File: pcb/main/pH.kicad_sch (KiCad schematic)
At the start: 12 parts

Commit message: fix: symbol libraries in Kicad 6.0
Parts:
- C1, C3: renamed from C?; value (none) -> 100n; footprint (none) -> Capacitor_SMD:C_0805_2012Metric_Pad1.15x1.40mm_HandSolder; symbol pHMeter-rescue:C-Device -> Device:C
- C9: renamed from C?; value (none) -> 22u; footprint (none) -> Capacitor_SMD:C_0805_2012Metric_Pad1.15x1.40mm_HandSolder; symbol pHMeter-rescue:C-Device -> Device:C
- J3: renamed from J?; symbol pHMeter-rescue:Conn_Coaxial_Power-Connector -> Connector:Conn_Coaxial_Power
- R11: renamed from R?; value (none) -> 56.2k; footprint (none) -> Resistor_SMD:R_0805_2012Metric_Pad1.15x1.40mm_HandSolder; symbol pHMeter-rescue:R-Device -> Device:R
- R13, R3, R4: renamed from R?; value (none) -> 10k; footprint (none) -> Resistor_SMD:R_0805_2012Metric_Pad1.15x1.40mm_HandSolder; symbol pHMeter-rescue:R-Device -> Device:R
- U1: renamed from U?; value (none) -> TLV6004PW; footprint (none) -> Package_SO:TSSOP-14_4.4x5mm_P0.65mm
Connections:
- net GND: now also C1.2, C3.2, C9.2, R4.2
- net Vin: now also C1.1, R3.2
- net pH+: now also C9.1, R11.1, R13.2
- net pH-: now also R13.1
- net at U1.3 (+), U1.5 (+): now also C3.1, R3.1, R4.1
- net at U1.10 (+): now also J3.1 (In)
- net at U1.8, U1.9 (-): now also R11.2
- net at U1.1, U1.2 (-): now also J3.2 (Ext)

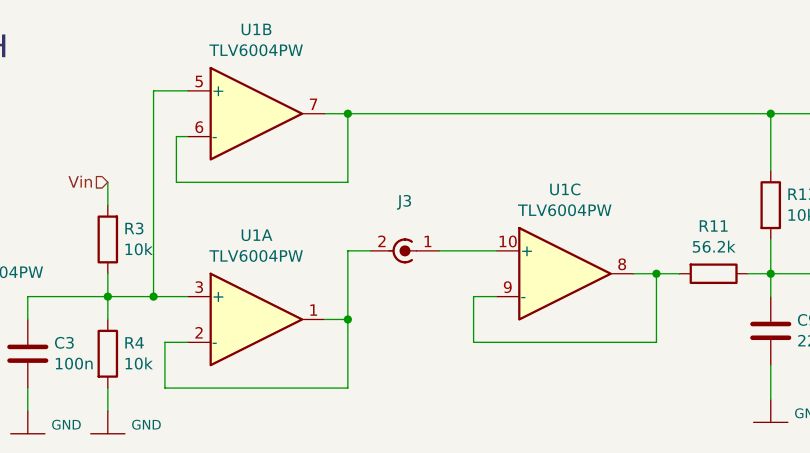
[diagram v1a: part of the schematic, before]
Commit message: fix: 3D model libraries in Kicad 6.0
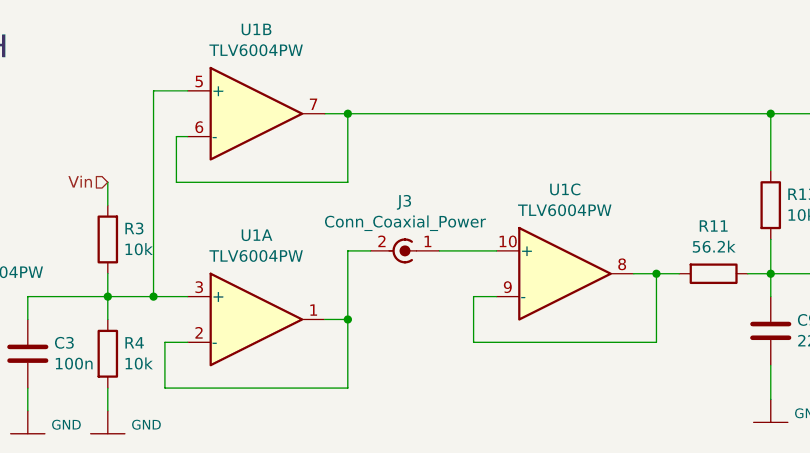
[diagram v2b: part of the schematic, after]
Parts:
- J3: value (none) -> Conn_Coaxial_Power; footprint (none) -> Connector_Coaxial:BNC_TEConnectivity_1478204_Vertical
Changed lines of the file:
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@@
     (in_bom yes) (on_board yes)
     (property "Reference" "J3" (id 0) (at 157.48 97.3582 90))
-    (property "Value" "" (id 1) (at 157.48 99.6696 90))
-    (property "Footprint" "" (id 2) (at 157.48 102.87 0)
+    (property "Value" "Conn_Coaxial_Power" (id 1) (at 157.48 99.6696 90))
+    (property "Footprint" "Connector_Coaxial:BNC_TEConnectivity_1478204_Vertical" (id 2) (at 157.48 102.87 0)
       (effects (font (size 1.27 1.27)) hide)
     )

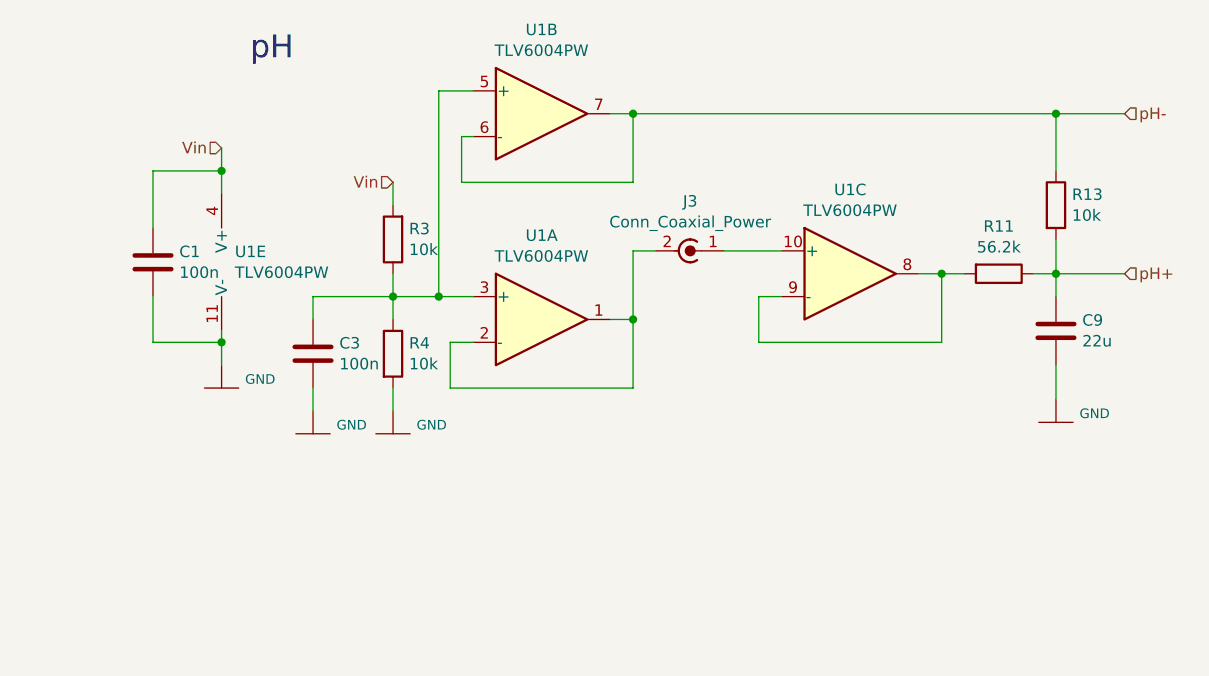
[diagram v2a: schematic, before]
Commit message: fix: standard footprint for R and C, BOM updated
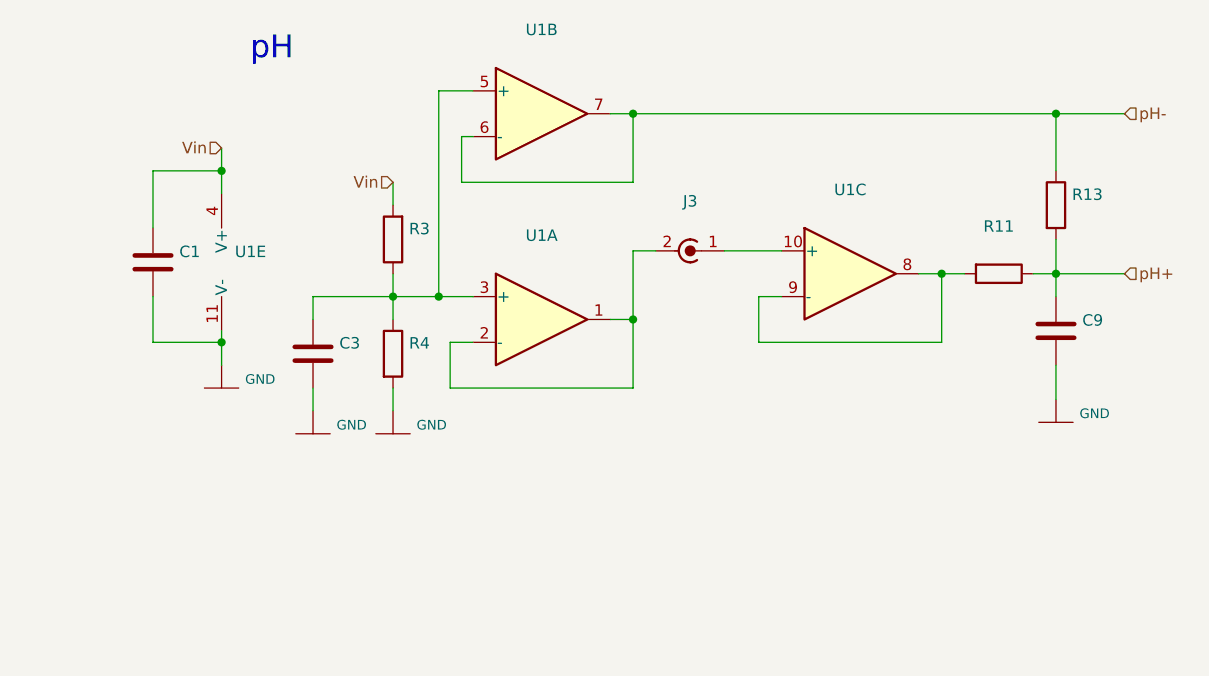
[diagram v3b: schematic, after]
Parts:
- C1, C3: value 100n -> (none); footprint Capacitor_SMD:C_0805_2012Metric_Pad1.15x1.40mm_HandSolder -> (none)
- C9: value 22u -> (none); footprint Capacitor_SMD:C_0805_2012Metric_Pad1.15x1.40mm_HandSolder -> (none)
- J3: value Conn_Coaxial_Power -> (none); footprint Connector_Coaxial:BNC_TEConnectivity_1478204_Vertical -> (none)
- R11: value 56.2k -> (none); footprint Resistor_SMD:R_0805_2012Metric_Pad1.15x1.40mm_HandSolder -> (none)
- R13, R3, R4: value 10k -> (none); footprint Resistor_SMD:R_0805_2012Metric_Pad1.15x1.40mm_HandSolder -> (none)
- U1: value TLV6004PW -> (none); footprint Package_SO:TSSOP-14_4.4x5mm_P0.65mm -> (none)
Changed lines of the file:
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@@
     (in_bom yes) (on_board yes)
     (property "Reference" "U1" (id 0) (at 140.97 78.3082 0))
-    (property "Value" "TLV6004PW" (id 1) (at 140.97 80.6196 0))
-    (property "Footprint" "Package_SO:TSSOP-14_4.4x5mm_P0.65mm" (id 2) (at 140.97 87.63 0)
+    (property "Value" "" (id 1) (at 140.97 80.6196 0))
+    (property "Footprint" "" (id 2) (at 140.97 87.63 0)
       (effects (font (size 1.27 1.27)) hide)
     )
@@
       (effects (font (size 1.27 1.27)) (justify left))
     )
-    (property "Value" "100n" (id 1) (at 118.491 115.443 0)
-      (effects (font (size 1.27 1.27)) (justify left))
-    )
-    (property "Footprint" "Capacitor_SMD:C_0805_2012Metric_Pad1.15x1.40mm_HandSolder" (id 2) (at 116.5352 118.11 0)
+    (property "Value" "" (id 1) (at 118.491 115.443 0)
+      (effects (font (size 1.27 1.27)) (justify left))
+    )
+    (property "Footprint" "" (id 2) (at 116.5352 118.11 0)
       (effects (font (size 1.27 1.27)) hide)
     )
@@
       (effects (font (size 1.27 1.27)) (justify right))
     )
-    (property "Value" "10k" (id 1) (at 126.238 102.743 0)
+    (property "Value" "" (id 1) (at 126.238 102.743 0)
       (effects (font (size 1.27 1.27)) (justify right))
     )
-    (property "Footprint" "Resistor_SMD:R_0805_2012Metric_Pad1.15x1.40mm_HandSolder" (id 2) (at 126.238 101.6 90)
+    (property "Footprint" "" (id 2) (at 126.238 101.6 90)
       (effects (font (size 1.27 1.27)) hide)
     )
@@
     (in_bom yes) (on_board yes)
     (property "Reference" "J3" (id 0) (at 157.48 97.3582 90))
-    (property "Value" "Conn_Coaxial_Power" (id 1) (at 157.48 99.6696 90))
-    (property "Footprint" "Connector_Coaxial:BNC_TEConnectivity_1478204_Vertical" (id 2) (at 157.48 102.87 0)
+    (property "Value" "" (id 1) (at 157.48 99.6696 90))
+    (property "Footprint" "" (id 2) (at 157.48 102.87 0)
       (effects (font (size 1.27 1.27)) hide)
     )
@@
     (in_bom yes) (on_board yes)
     (property "Reference" "U1" (id 0) (at 175.26 96.0882 0))
-    (property "Value" "TLV6004PW" (id 1) (at 175.26 98.3996 0))
-    (property "Footprint" "Package_SO:TSSOP-14_4.4x5mm_P0.65mm" (id 2) (at 175.26 105.41 0)
+    (property "Value" "" (id 1) (at 175.26 98.3996 0))
+    (property "Footprint" "" (id 2) (at 175.26 105.41 0)
       (effects (font (size 1.27 1.27)) hide)
     )
@@
     (in_bom yes) (on_board yes)
     (property "Reference" "R11" (id 0) (at 191.77 100.1522 90))
-    (property "Value" "56.2k" (id 1) (at 191.77 102.4636 90))
-    (property "Footprint" "Resistor_SMD:R_0805_2012Metric_Pad1.15x1.40mm_HandSolder" (id 2) (at 191.77 103.632 90)
+    (property "Value" "" (id 1) (at 191.77 102.4636 90))
+    (property "Footprint" "" (id 2) (at 191.77 103.632 90)
       (effects (font (size 1.27 1.27)) hide)
     )
@@
       (effects (font (size 1.27 1.27)) (justify left))
     )
-    (property "Value" "10k" (id 1) (at 199.898 98.933 0)
-      (effects (font (size 1.27 1.27)) (justify left))
-    )
-    (property "Footprint" "Resistor_SMD:R_0805_2012Metric_Pad1.15x1.40mm_HandSolder" (id 2) (at 196.342 97.79 90)
+    (property "Value" "" (id 1) (at 199.898 98.933 0)
+      (effects (font (size 1.27 1.27)) (justify left))
+    )
+    (property "Footprint" "" (id 2) (at 196.342 97.79 90)
       (effects (font (size 1.27 1.27)) hide)
     )
@@
       (effects (font (size 1.27 1.27)) (justify left))
     )
-    (property "Value" "22u" (id 1) (at 201.041 112.903 0)
-      (effects (font (size 1.27 1.27)) (justify left))
-    )
-    (property "Footprint" "Capacitor_SMD:C_0805_2012Metric_Pad1.15x1.40mm_HandSolder" (id 2) (at 199.0852 115.57 0)
+    (property "Value" "" (id 1) (at 201.041 112.903 0)
+      (effects (font (size 1.27 1.27)) (justify left))
+    )
+    (property "Footprint" "" (id 2) (at 199.0852 115.57 0)
       (effects (font (size 1.27 1.27)) hide)
     )
@@
       (effects (font (size 1.27 1.27)) (justify left))
     )
-    (property "Value" "TLV6004PW" (id 1) (at 106.8832 105.283 0)
-      (effects (font (size 1.27 1.27)) (justify left))
-    )
-    (property "Footprint" "Package_SO:TSSOP-14_4.4x5mm_P0.65mm" (id 2) (at 107.95 104.14 0)
+    (property "Value" "" (id 1) (at 106.8832 105.283 0)
+      (effects (font (size 1.27 1.27)) (justify left))
+    )
+    (property "Footprint" "" (id 2) (at 107.95 104.14 0)
       (effects (font (size 1.27 1.27)) hide)
     )
@@
       (effects (font (size 1.27 1.27)) (justify left))
     )
-    (property "Value" "100n" (id 1) (at 100.711 105.283 0)
-      (effects (font (size 1.27 1.27)) (justify left))
-    )
-    (property "Footprint" "Capacitor_SMD:C_0805_2012Metric_Pad1.15x1.40mm_HandSolder" (id 2) (at 98.7552 107.95 0)
+    (property "Value" "" (id 1) (at 100.711 105.283 0)
+      (effects (font (size 1.27 1.27)) (justify left))
+    )
+    (property "Footprint" "" (id 2) (at 98.7552 107.95 0)
       (effects (font (size 1.27 1.27)) hide)
     )
@@
     (in_bom yes) (on_board yes)
     (property "Reference" "U1" (id 0) (at 140.97 101.1682 0))
-    (property "Value" "TLV6004PW" (id 1) (at 140.97 103.4796 0))
-    (property "Footprint" "Package_SO:TSSOP-14_4.4x5mm_P0.65mm" (id 2) (at 140.97 110.49 0)
+    (property "Value" "" (id 1) (at 140.97 103.4796 0))
+    (property "Footprint" "" (id 2) (at 140.97 110.49 0)
       (effects (font (size 1.27 1.27)) hide)
     )
@@
       (effects (font (size 1.27 1.27)) (justify left))
     )
-    (property "Value" "10k" (id 1) (at 126.238 115.443 0)
-      (effects (font (size 1.27 1.27)) (justify left))
-    )
-    (property "Footprint" "Resistor_SMD:R_0805_2012Metric_Pad1.15x1.40mm_HandSolder" (id 2) (at 122.682 114.3 90)
-      (effects (font (size 1.27 1.27)) hide)
-    )
+    (property "Value" "" (id 1) (at 126.238 115.443 0)
+      (effects (font (size 1.27 1.27)) (justify left))
+    )
+    (property "Footprint" "" (id 2) (at 122.682 114.3 90)
+      (effects (font (size 1.27 1.27)) hide)
+    )

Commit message: feat: updated BOM
BOM ready to order in v0.2
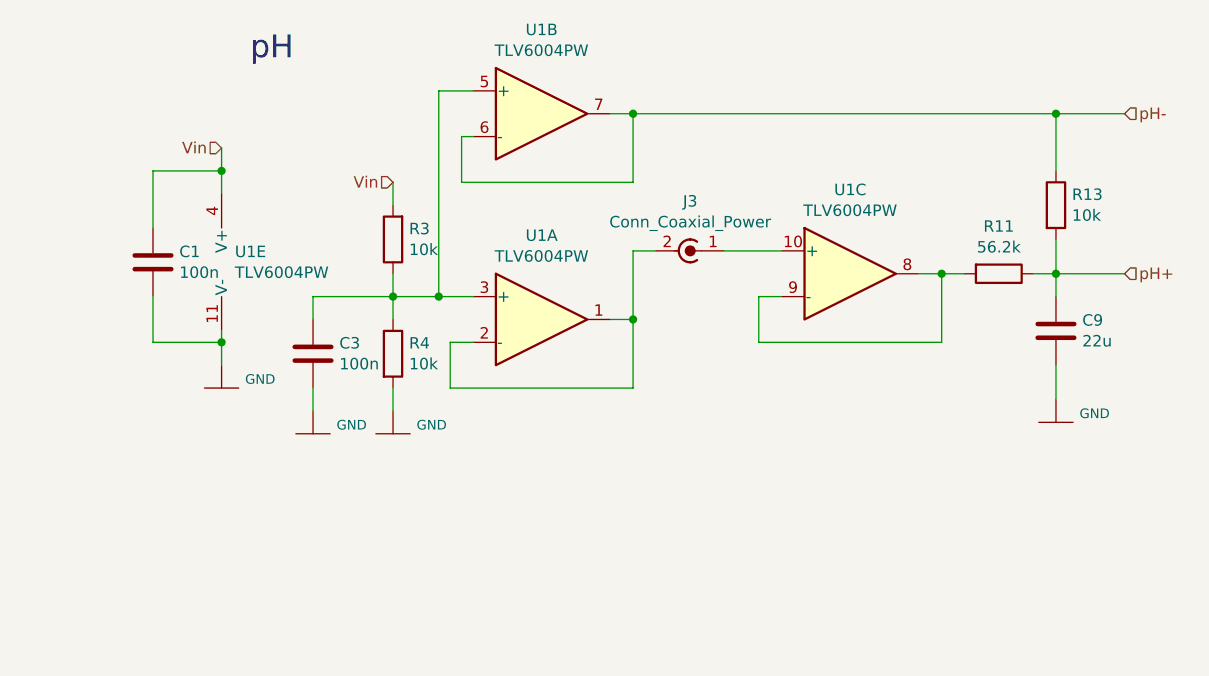
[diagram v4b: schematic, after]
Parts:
- C1, C3: value (none) -> 100n; footprint (none) -> Capacitor_SMD:C_0805_2012Metric_Pad1.18x1.45mm_HandSolder
- C9: value (none) -> 22u; footprint (none) -> Capacitor_SMD:C_0805_2012Metric_Pad1.15x1.40mm_HandSolder
- J3: value (none) -> Conn_Coaxial_Power; footprint (none) -> Connector_Coaxial:BNC_TEConnectivity_1478204_Vertical
- R11: value (none) -> 56.2k; footprint (none) -> Resistor_SMD:R_0805_2012Metric_Pad1.15x1.40mm_HandSolder
- R13, R3, R4: value (none) -> 10k; footprint (none) -> Resistor_SMD:R_0805_2012Metric_Pad1.20x1.40mm_HandSolder
- U1: value (none) -> TLV6004PW; footprint (none) -> Package_SO:TSSOP-14_4.4x5mm_P0.65mm

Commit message: feat: update sch
Schematic updated with new BOM
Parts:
- R11: MFN (none) -> YAGEO; MFP (none) -> RC0805FR-0756K2L; S1PL (none) -> https://www.mouser.com/ProductDetail/YAGEO/RC0805FR-0756K2L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; S1PN (none) -> 603-RC0805FR-0756K2L
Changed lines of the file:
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@@
       (effects (font (size 1.27 1.27)) hide)
     )
-    (property "Datasheet" "~" (id 3) (at 191.77 105.41 0)
+    (property "Datasheet" "https://www.mouser.com/datasheet/2/447/Yageo_03_18_2021_PYu_RC_Group_51_RoHS_L_11-2199992.pdf" (id 3) (at 191.77 105.41 0)
       (effects (font (size 1.27 1.27)) hide)
     )
+    (property "Description" "Resistores de película gruesa - SMD 56.2 kOhms 125 mW 0805 1% " (id 4) (at 191.77 105.41 0)
+      (effects (font (size 1.27 1.27)) hide)
+    )
+    (property "MFN" "YAGEO" (id 5) (at 191.77 105.41 0)
+      (effects (font (size 1.27 1.27)) hide)
+    )
+    (property "MFP" "RC0805FR-0756K2L" (id 6) (at 191.77 105.41 0)
+      (effects (font (size 1.27 1.27)) hide)
+    )
+    (property "S1PL" "https://www.mouser.com/ProductDetail/YAGEO/RC0805FR-0756K2L?qs=sGAEpiMZZMtlubZbdhIBIDa%2FhYjOd3Y%252BVOG828%2F3Oq8%3D" (id 7) (at 191.77 105.41 0)
+      (effects (font (size 1.27 1.27)) hide)
+    )
+    (property "S1PN" "603-RC0805FR-0756K2L " (id 8) (at 191.77 105.41 0)
+      (effects (font (size 1.27 1.27)) hide)
+    )

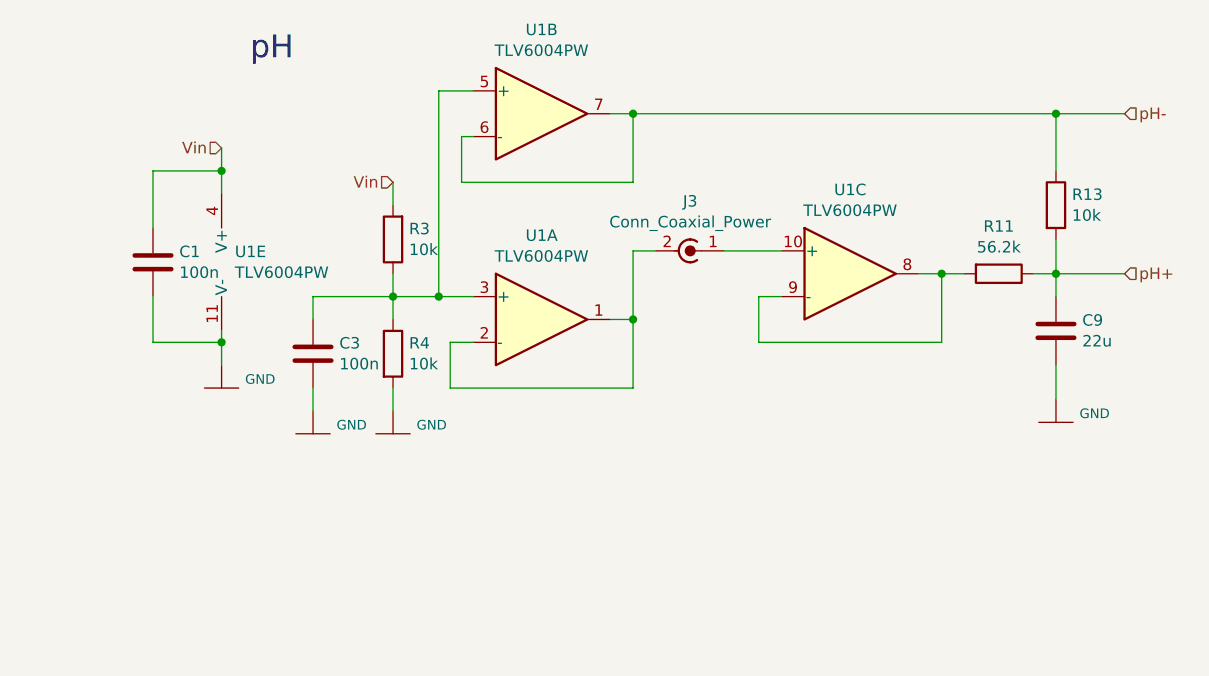
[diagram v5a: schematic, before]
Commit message: feat: new PCB version to 1.1.2
Schematic:
- Updated sheets to 1.1.2 version.
- Change inputs for last OPA in EC sheet.
- INA- and INA+ set to GND in 24bits sheet for reduce noise.
- Change /CE connection (TX -> HWB) in Memory and COMM LED.
- Adding a correct guard in pH sheet.
- Adding correct 12 V support for 3.3 V (avoid battery charge circuit).

Design:
- Increase width track for 2 A in 3.3 V power supply.
- Order labels.
- Put new schottky diode for 12 V -> 3.3 V circuit direct connection.
- Adding pH and EC tag.
- Adding guard and restrict area for pH adquisiton.
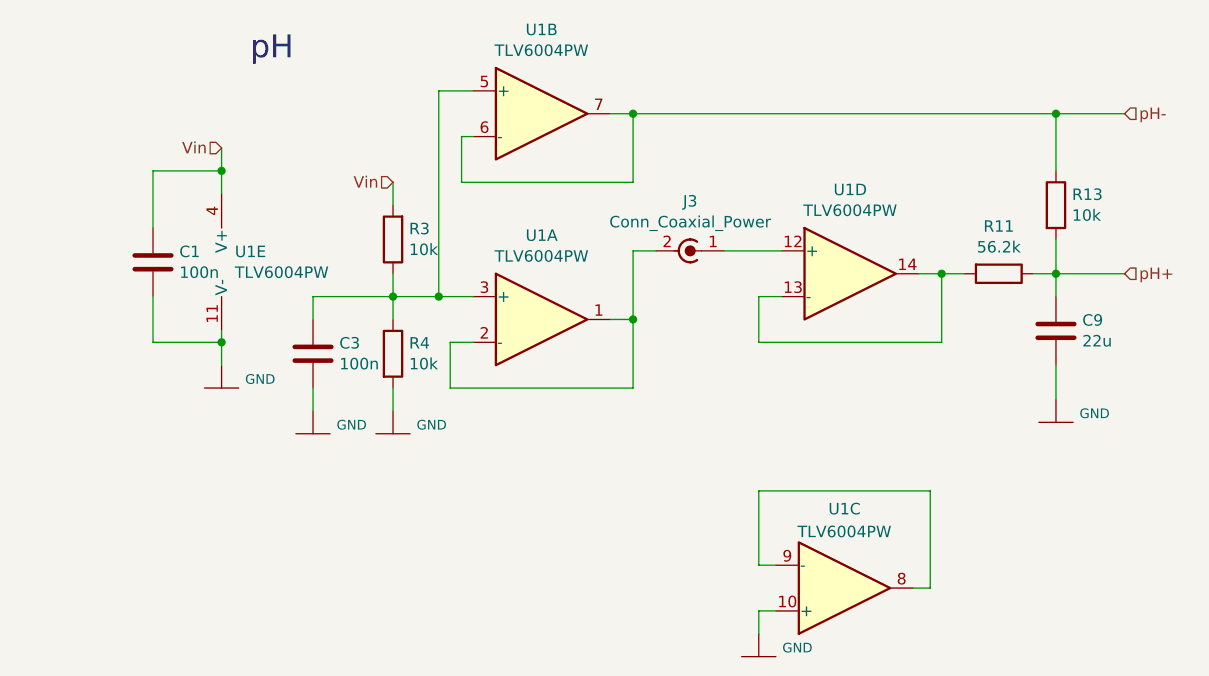
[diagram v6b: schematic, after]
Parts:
- added unit 3 of U1
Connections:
- net GND: now also U1.10 (+)
- net at J3.1 (In): now also U1.12 (+); no longer U1.10 (+)
- new net: R11.2, U1.13 (-), U1.14
- new net: U1.8, U1.9 (-)
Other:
- company: (none) -> Hackuarium
- title: (none) -> pH Adquisition
